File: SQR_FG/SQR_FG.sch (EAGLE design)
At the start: 24 parts, among them IC1 MEGA328P, IC2 NJM7032, Q1 16MHz, SW1 EC12E_SW

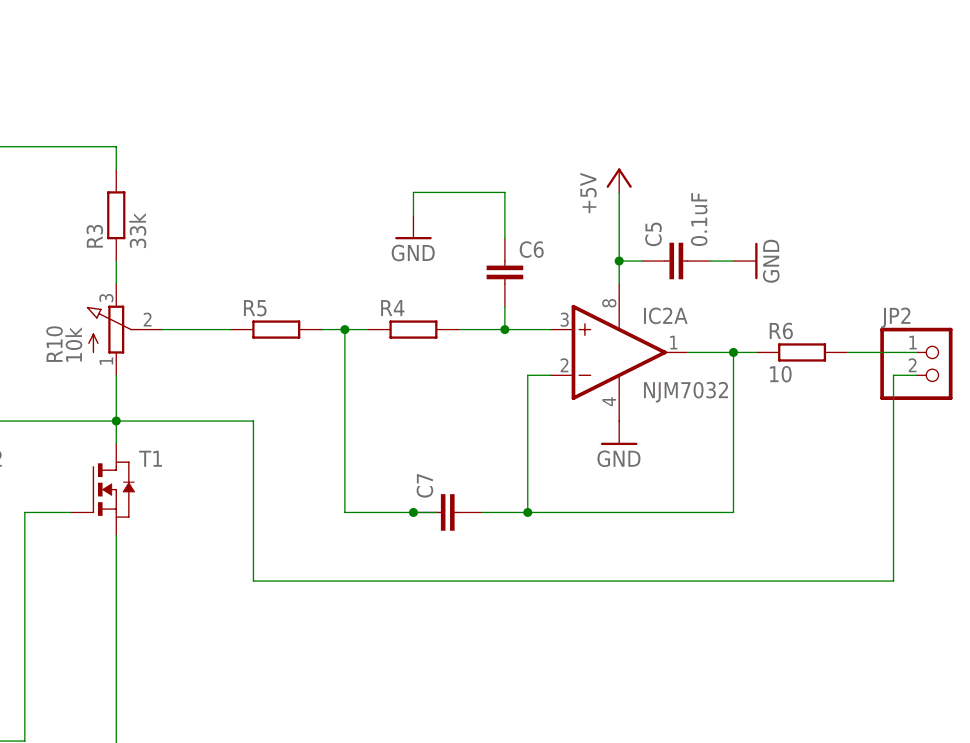
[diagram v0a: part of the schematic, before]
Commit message: SQR_FG Bypass by C
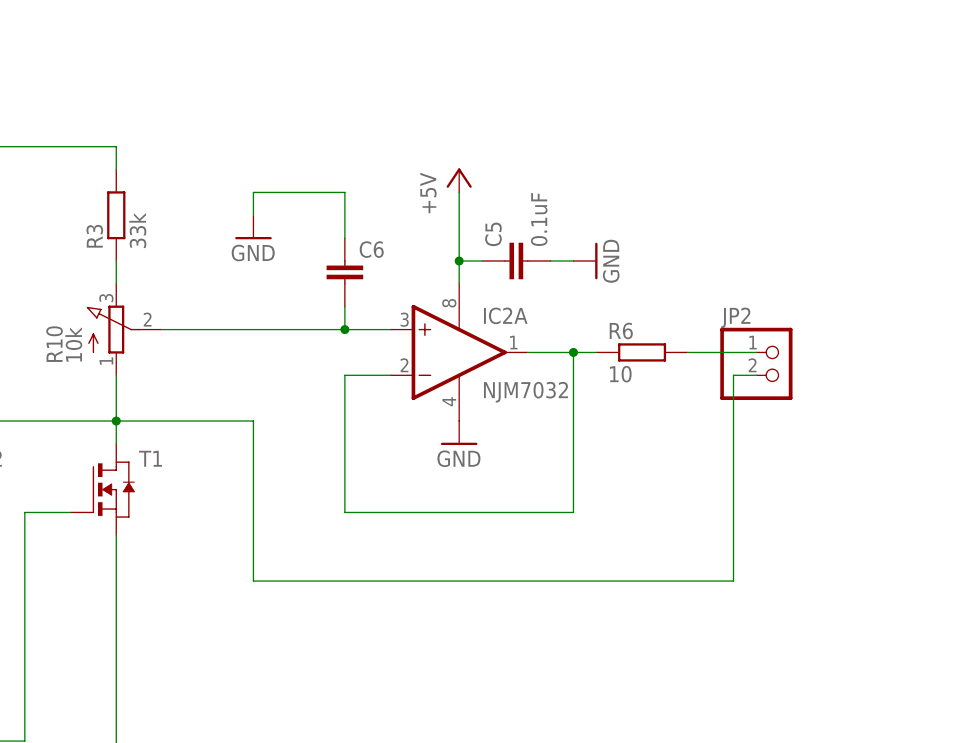
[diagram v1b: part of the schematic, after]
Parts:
- removed C7: (no value), rcl:C-EU025-024X044
- removed R4, R5: (no value), rcl:R-EU_0207/7
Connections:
- removed net N$14: C6.2, IC2A.+IN, R4.2
- removed net N$4: C7.1, R4.1, R5.2
- net N$15: now also C6.2, IC2A.+IN; no longer R5.1
- net N$16: no longer C7.2
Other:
- moved on the sheet: C5, C6, IC2A, JP2, R6
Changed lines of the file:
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@@
 <part name="JP2" library="pinhead" deviceset="PINHD-1X2" device=""/>
 <part name="R3" library="rcl" deviceset="R-EU_" device="0207/7" value="33k"/>
-<part name="R4" library="rcl" deviceset="R-EU_" device="0207/7"/>
-<part name="R5" library="rcl" deviceset="R-EU_" device="0207/7"/>
 <part name="C6" library="rcl" deviceset="C-EU" device="025-024X044"/>
-<part name="C7" library="rcl" deviceset="C-EU" device="025-024X044"/>
 <part name="GND6" library="supply1" deviceset="GND" device=""/>
 </parts>
@@
 <instance part="SW1" gate="G$2" x="132.08" y="73.66"/>
 <instance part="GND4" gate="1" x="139.7" y="63.5"/>
-<instance part="P+3" gate="1" x="238.76" y="114.3"/>
-<instance part="GND7" gate="1" x="238.76" y="83.82"/>
-<instance part="IC2" gate="A" x="238.76" y="93.98"/>
+<instance part="P+3" gate="1" x="220.98" y="114.3"/>
+<instance part="GND7" gate="1" x="220.98" y="83.82"/>
+<instance part="IC2" gate="A" x="220.98" y="93.98"/>
 <instance part="IC2" gate="B" x="162.56" y="27.94"/>
-<instance part="IC2" gate="P" x="238.76" y="93.98"/>
-<instance part="R6" gate="G$1" x="259.08" y="93.98"/>
+<instance part="IC2" gate="P" x="220.98" y="93.98"/>
+<instance part="R6" gate="G$1" x="241.3" y="93.98"/>
 <instance part="R7" gate="G$1" x="139.7" y="38.1" rot="R90"/>
 <instance part="R8" gate="G$1" x="139.7" y="22.86" rot="R90"/>
@@
 <instance part="T2" gate="A" x="165.1" y="78.74"/>
 <instance part="GND10" gate="1" x="165.1" y="71.12"/>
-<instance part="C5" gate="G$1" x="243.84" y="104.14" rot="R90"/>
-<instance part="GND5" gate="1" x="254" y="104.14" rot="R90"/>
-<instance part="JP2" gate="G$1" x="274.32" y="91.44"/>
+<instance part="C5" gate="G$1" x="226.06" y="104.14" rot="R90"/>
+<instance part="GND5" gate="1" x="236.22" y="104.14" rot="R90"/>
+<instance part="JP2" gate="G$1" x="256.54" y="91.44"/>
 <instance part="R3" gate="G$1" x="182.88" y="109.22" rot="R90"/>
-<instance part="R4" gate="G$1" x="215.9" y="96.52"/>
-<instance part="R5" gate="G$1" x="200.66" y="96.52"/>
-<instance part="C6" gate="G$1" x="226.06" y="104.14"/>
-<instance part="C7" gate="G$1" x="218.44" y="76.2" rot="R90"/>
-<instance part="GND6" gate="1" x="215.9" y="106.68"/>
+<instance part="C6" gate="G$1" x="208.28" y="104.14"/>
+<instance part="GND6" gate="1" x="198.12" y="106.68"/>
 </instances>
 <busses>
@@
 <pinref part="C5" gate="G$1" pin="2"/>
 <pinref part="GND5" gate="1" pin="GND"/>
-<wire x1="251.46" y1="104.14" x2="248.92" y2="104.14" width="0.1524" layer="91"/>
+<wire x1="233.68" y1="104.14" x2="231.14" y2="104.14" width="0.1524" layer="91"/>
 </segment>
 <segment>
 <pinref part="C6" gate="G$1" pin="1"/>
-<wire x1="226.06" y1="106.68" x2="226.06" y2="111.76" width="0.1524" layer="91"/>
-<wire x1="226.06" y1="111.76" x2="215.9" y2="111.76" width="0.1524" layer="91"/>
+<wire x1="208.28" y1="106.68" x2="208.28" y2="111.76" width="0.1524" layer="91"/>
+<wire x1="208.28" y1="111.76" x2="198.12" y2="111.76" width="0.1524" layer="91"/>
 <pinref part="GND6" gate="1" pin="GND"/>
-<wire x1="215.9" y1="111.76" x2="215.9" y2="109.22" width="0.1524" layer="91"/>
+<wire x1="198.12" y1="111.76" x2="198.12" y2="109.22" width="0.1524" layer="91"/>
 </segment>
 </net>
@@
 <segment>
 <pinref part="IC2" gate="P" pin="V+"/>
-<wire x1="238.76" y1="101.6" x2="238.76" y2="104.14" width="0.1524" layer="91"/>
+<wire x1="220.98" y1="101.6" x2="220.98" y2="104.14" width="0.1524" layer="91"/>
 <pinref part="P+3" gate="1" pin="+5V"/>
 <pinref part="C5" gate="G$1" pin="1"/>
-<wire x1="238.76" y1="104.14" x2="238.76" y2="111.76" width="0.1524" layer="91"/>
-<wire x1="241.3" y1="104.14" x2="238.76" y2="104.14" width="0.1524" layer="91"/>
-<junction x="238.76" y="104.14"/>
+<wire x1="220.98" y1="104.14" x2="220.98" y2="111.76" width="0.1524" layer="91"/>
+<wire x1="223.52" y1="104.14" x2="220.98" y2="104.14" width="0.1524" layer="91"/>
+<junction x="220.98" y="104.14"/>
 </segment>
 </net>
@@
 <net name="N$16" class="0">
 <segment>
-<wire x1="231.14" y1="91.44" x2="228.6" y2="91.44" width="0.1524" layer="91"/>
-<wire x1="228.6" y1="91.44" x2="228.6" y2="76.2" width="0.1524" layer="91"/>
-<wire x1="228.6" y1="76.2" x2="251.46" y2="76.2" width="0.1524" layer="91"/>
-<wire x1="251.46" y1="76.2" x2="251.46" y2="93.98" width="0.1524" layer="91"/>
-<wire x1="251.46" y1="93.98" x2="246.38" y2="93.98" width="0.1524" layer="91"/>
+<wire x1="213.36" y1="91.44" x2="208.28" y2="91.44" width="0.1524" layer="91"/>
+<wire x1="208.28" y1="91.44" x2="208.28" y2="76.2" width="0.1524" layer="91"/>
+<wire x1="208.28" y1="76.2" x2="233.68" y2="76.2" width="0.1524" layer="91"/>
+<wire x1="233.68" y1="76.2" x2="233.68" y2="93.98" width="0.1524" layer="91"/>
+<wire x1="233.68" y1="93.98" x2="228.6" y2="93.98" width="0.1524" layer="91"/>
 <pinref part="IC2" gate="A" pin="-IN"/>
 <pinref part="IC2" gate="A" pin="OUT"/>
 <pinref part="R6" gate="G$1" pin="1"/>
-<wire x1="254" y1="93.98" x2="251.46" y2="93.98" width="0.1524" layer="91"/>
-<junction x="251.46" y="93.98"/>
-<pinref part="C7" gate="G$1" pin="2"/>
-<wire x1="223.52" y1="76.2" x2="228.6" y2="76.2" width="0.1524" layer="91"/>
-<junction x="228.6" y="76.2"/>
+<wire x1="236.22" y1="93.98" x2="233.68" y2="93.98" width="0.1524" layer="91"/>
+<junction x="233.68" y="93.98"/>
 </segment>
 </net>
@@
 <segment>
 <pinref part="R6" gate="G$1" pin="2"/>
-<wire x1="264.16" y1="93.98" x2="271.78" y2="93.98" width="0.1524" layer="91"/>
+<wire x1="246.38" y1="93.98" x2="254" y2="93.98" width="0.1524" layer="91"/>
 <pinref part="JP2" gate="G$1" pin="1"/>
 </segment>
@@
 <wire x1="182.88" y1="86.36" x2="198.12" y2="86.36" width="0.1524" layer="91"/>
 <wire x1="198.12" y1="86.36" x2="198.12" y2="68.58" width="0.1524" layer="91"/>
-<wire x1="198.12" y1="68.58" x2="269.24" y2="68.58" width="0.1524" layer="91"/>
-<wire x1="269.24" y1="68.58" x2="269.24" y2="91.44" width="0.1524" layer="91"/>
+<wire x1="198.12" y1="68.58" x2="251.46" y2="68.58" width="0.1524" layer="91"/>
+<wire x1="251.46" y1="68.58" x2="251.46" y2="91.44" width="0.1524" layer="91"/>
 <pinref part="JP2" gate="G$1" pin="2"/>
-<wire x1="271.78" y1="91.44" x2="269.24" y2="91.44" width="0.1524" layer="91"/>
+<wire x1="254" y1="91.44" x2="251.46" y2="91.44" width="0.1524" layer="91"/>
 </segment>
 </net>
@@
 </segment>
 </net>
-<net name="N$4" class="0">
-<segment>
-<pinref part="R5" gate="G$1" pin="2"/>
-<pinref part="R4" gate="G$1" pin="1"/>
-<wire x1="205.74" y1="96.52" x2="208.28" y2="96.52" width="0.1524" layer="91"/>
-<wire x1="208.28" y1="96.52" x2="210.82" y2="96.52" width="0.1524" layer="91"/>
-<wire x1="218.44" y1="76.2" x2="215.9" y2="76.2" width="0.1524" layer="91"/>
-<wire x1="215.9" y1="76.2" x2="208.28" y2="76.2" width="0.1524" layer="91"/>
-<wire x1="208.28" y1="76.2" x2="208.28" y2="96.52" width="0.1524" layer="91"/>
+<net name="N$15" class="0">
+<segment>
+<wire x1="187.96" y1="96.52" x2="208.28" y2="96.52" width="0.1524" layer="91"/>
+<pinref part="IC2" gate="A" pin="+IN"/>
+<pinref part="C6" gate="G$1" pin="2"/>
+<wire x1="208.28" y1="96.52" x2="213.36" y2="96.52" width="0.1524" layer="91"/>
+<wire x1="208.28" y1="99.06" x2="208.28" y2="96.52" width="0.1524" layer="91"/>
 <junction x="208.28" y="96.52"/>
-<pinref part="C7" gate="G$1" pin="1"/>
-<junction x="215.9" y="76.2"/>
-</segment>
-</net>
-<net name="N$14" class="0">
-<segment>
-<pinref part="R4" gate="G$1" pin="2"/>
-<pinref part="IC2" gate="A" pin="+IN"/>
-<wire x1="220.98" y1="96.52" x2="226.06" y2="96.52" width="0.1524" layer="91"/>
-<pinref part="C6" gate="G$1" pin="2"/>
-<wire x1="226.06" y1="96.52" x2="231.14" y2="96.52" width="0.1524" layer="91"/>
-<wire x1="226.06" y1="99.06" x2="226.06" y2="96.52" width="0.1524" layer="91"/>
-<junction x="226.06" y="96.52"/>
-</segment>
-</net>
-<net name="N$15" class="0">
-<segment>
-<pinref part="R5" gate="G$1" pin="1"/>
-<wire x1="195.58" y1="96.52" x2="187.96" y2="96.52" width="0.1524" layer="91"/>
-</segment>
-</net>
+</segment>
+</net>
